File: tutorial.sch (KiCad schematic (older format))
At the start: 24 parts, among them SW1 SW_Push, U1 ATmega32U4-AU, Y1 16MHz

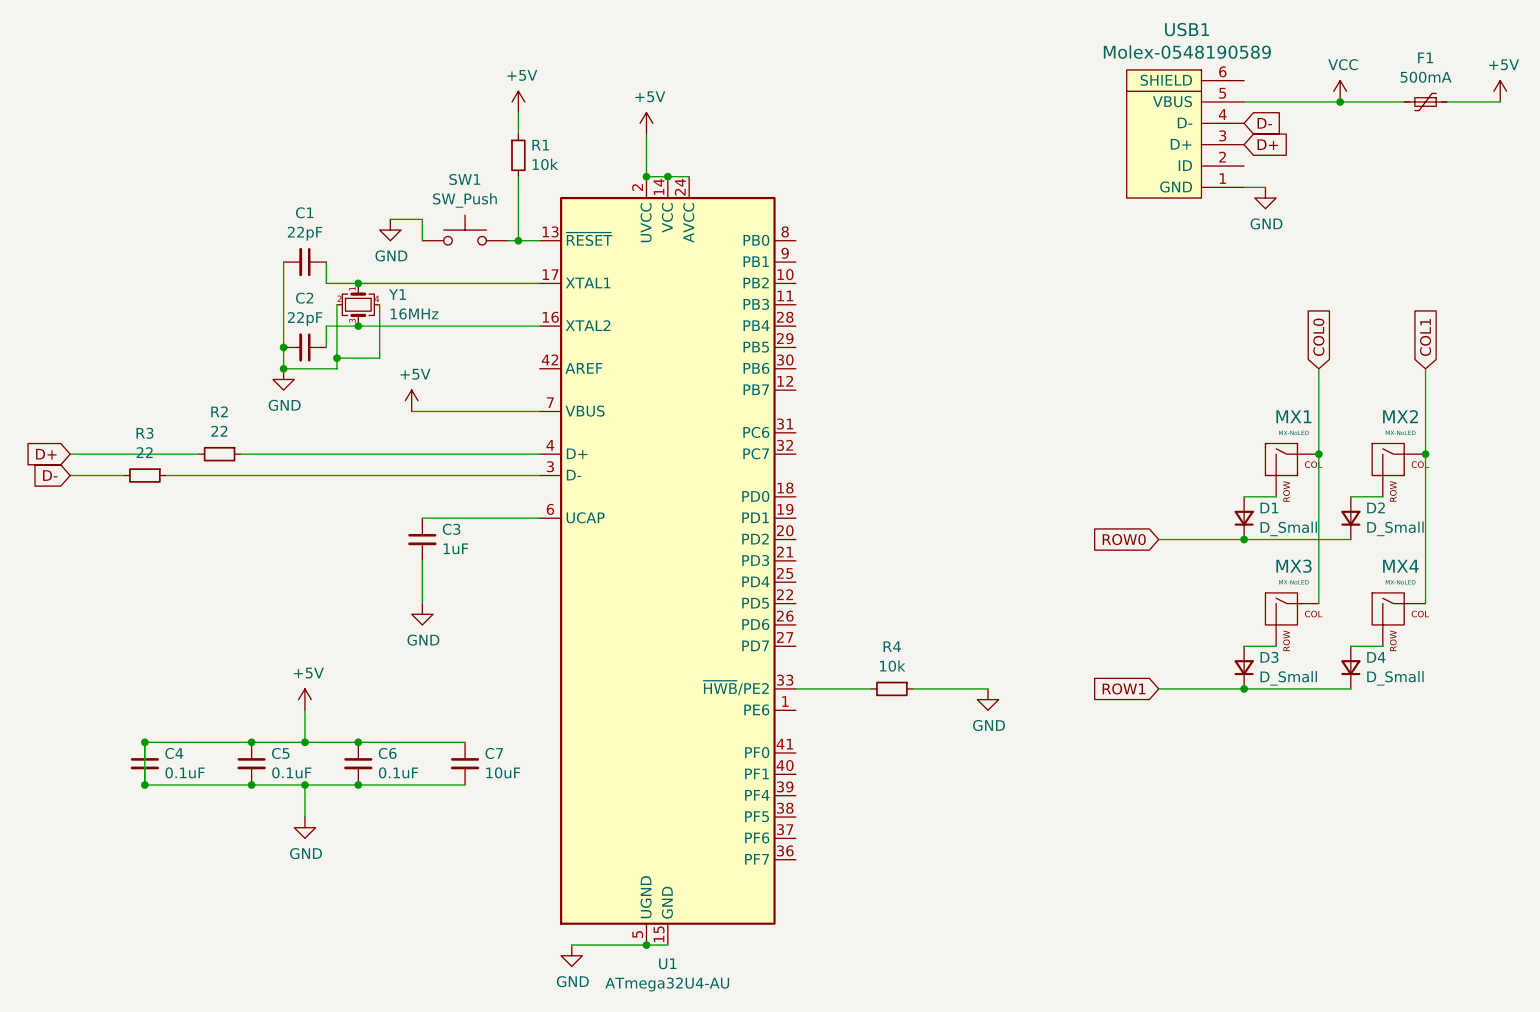
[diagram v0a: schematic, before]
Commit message: Fixes and cleanup
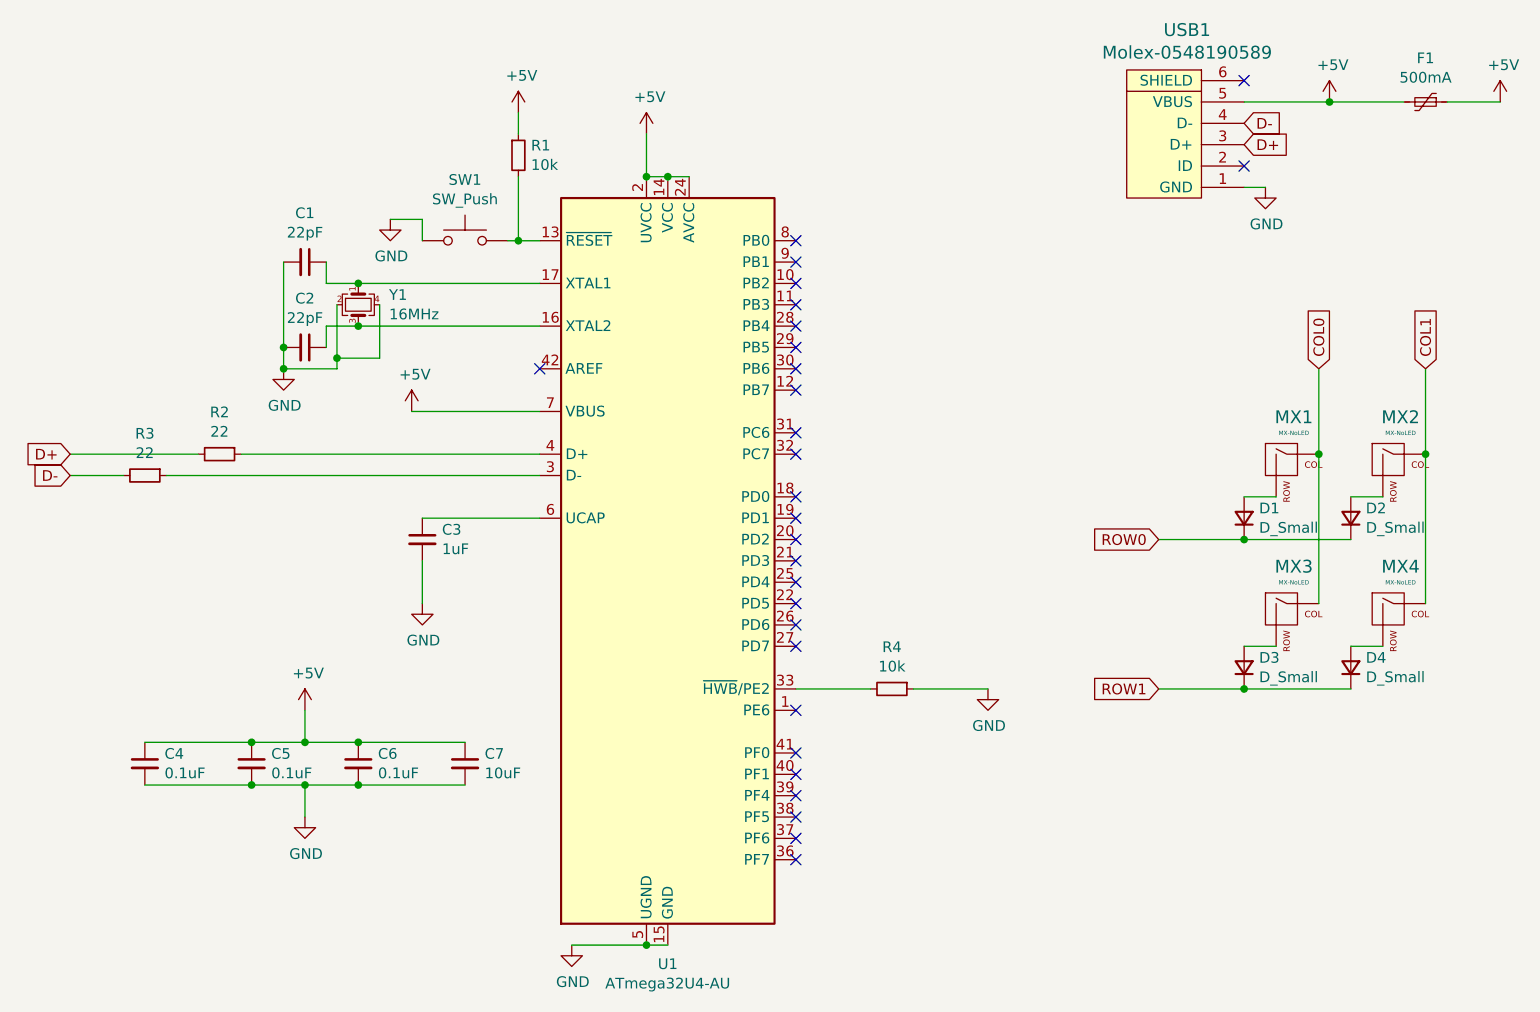
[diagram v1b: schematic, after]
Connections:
- net VCC is gone; now on net +5V: F1.2, USB1.5 (VBUS)
- net +5V: no longer C1.2, C2.2, C3.2, C4.2, C5.2, C6.2, C7.2, R4.1, SW1.1, U1.15 (GND), U1.23 (GND), U1.35 (GND), U1.43 (GND), U1.5 (UGND), USB1.1 (GND), Y1.2, Y1.4
- new net GND: C1.2, C2.2, C3.2, C4.2, C5.2, C6.2, C7.2, R4.1, SW1.1, U1.15 (GND), U1.23 (GND), U1.35 (GND), U1.43 (GND), U1.5 (UGND), USB1.1 (GND), Y1.2, Y1.4
- no-connect marks 0 -> 28

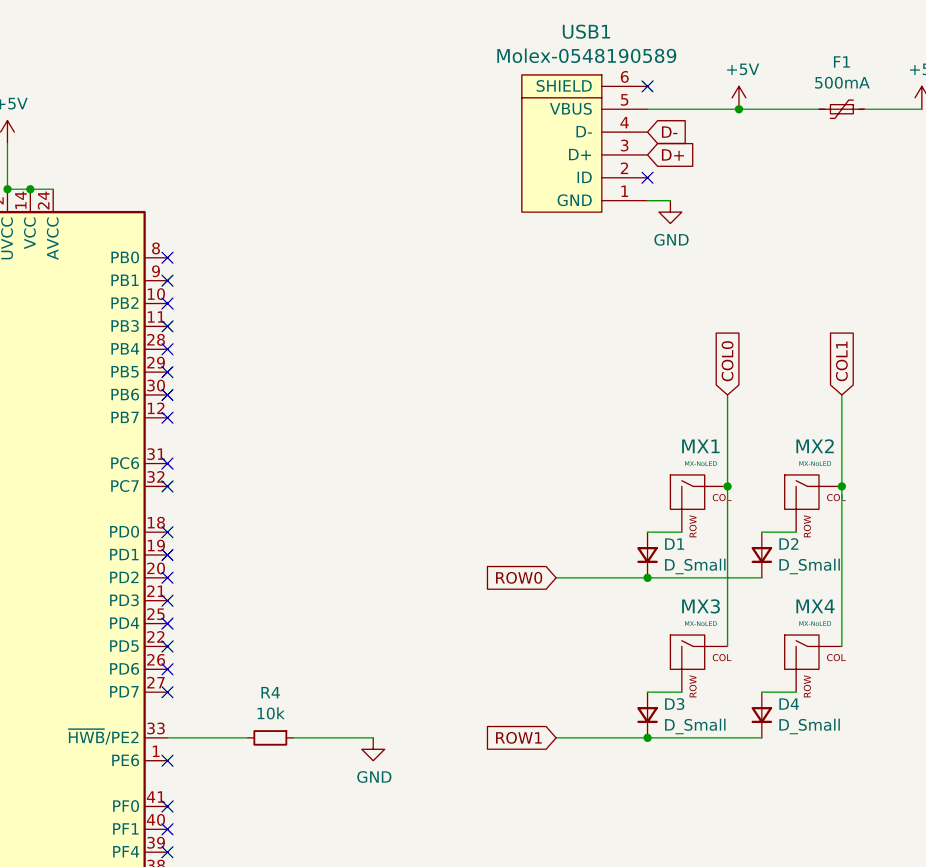
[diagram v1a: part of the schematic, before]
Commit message: Finished routing
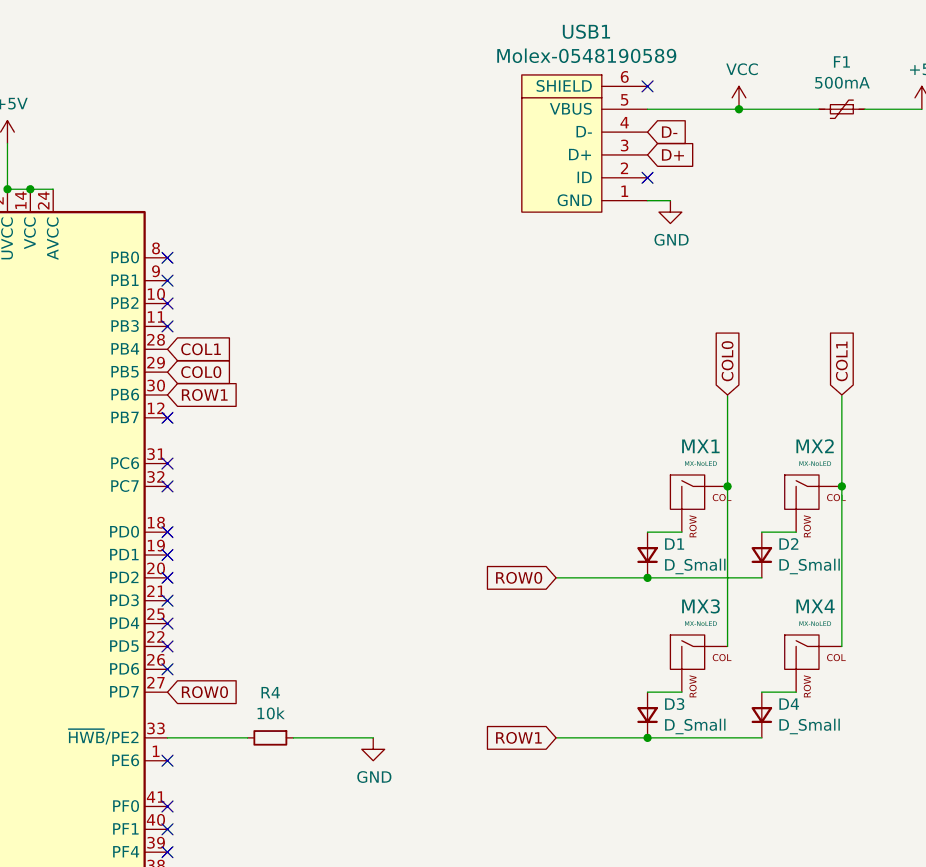
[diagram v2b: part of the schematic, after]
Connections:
- net +5V: no longer F1.2, USB1.5 (VBUS)
- net COL0: now also U1.29 (PB5)
- net COL1: now also U1.28 (PB4)
- net ROW0: now also U1.27 (PD7)
- net ROW1: now also U1.30 (PB6)
- new net VCC: F1.2, USB1.5 (VBUS)
- no-connect marks 28 -> 24
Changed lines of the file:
@@
 NoConn ~ 6550 4700
 NoConn ~ 6550 4500
-NoConn ~ 6550 4200
 NoConn ~ 6550 4100
 NoConn ~ 6550 4000
@@
 NoConn ~ 6550 3200
 NoConn ~ 6550 3000
-NoConn ~ 6550 2900
-NoConn ~ 6550 2800
-NoConn ~ 6550 2700
 NoConn ~ 6550 2600
 NoConn ~ 6550 2500
@@
 	8650 1650 9050 1650
 $Comp
-L power:+5V #PWR0111
-U 1 1 5F3DD71F
+L power:VCC #PWR?
+U 1 1 5F3E01DE
 P 9050 1650
-F 0 "#PWR0111" H 9050 1500 50  0001 C CNN
-F 1 "+5V" H 9065 1823 50  0000 C CNN
+F 0 "#PWR?" H 9050 1500 50  0001 C CNN
+F 1 "VCC" H 9065 1823 50  0000 C CNN
 F 2 "" H 9050 1650 50  0001 C CNN
 F 3 "" H 9050 1650 50  0001 C CNN
@@
 Wire Wire Line
 	9050 1650 9400 1650
+Text GLabel 6550 4200 2    50   Input ~ 0
+ROW0
+Text GLabel 6550 2900 2    50   Input ~ 0
+ROW1
+Text GLabel 6550 2700 2    50   Input ~ 0
+COL1
+Text GLabel 6550 2800 2    50   Input ~ 0
+COL0
 $EndSCHEMATC
